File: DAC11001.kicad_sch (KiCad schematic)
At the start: 5 parts

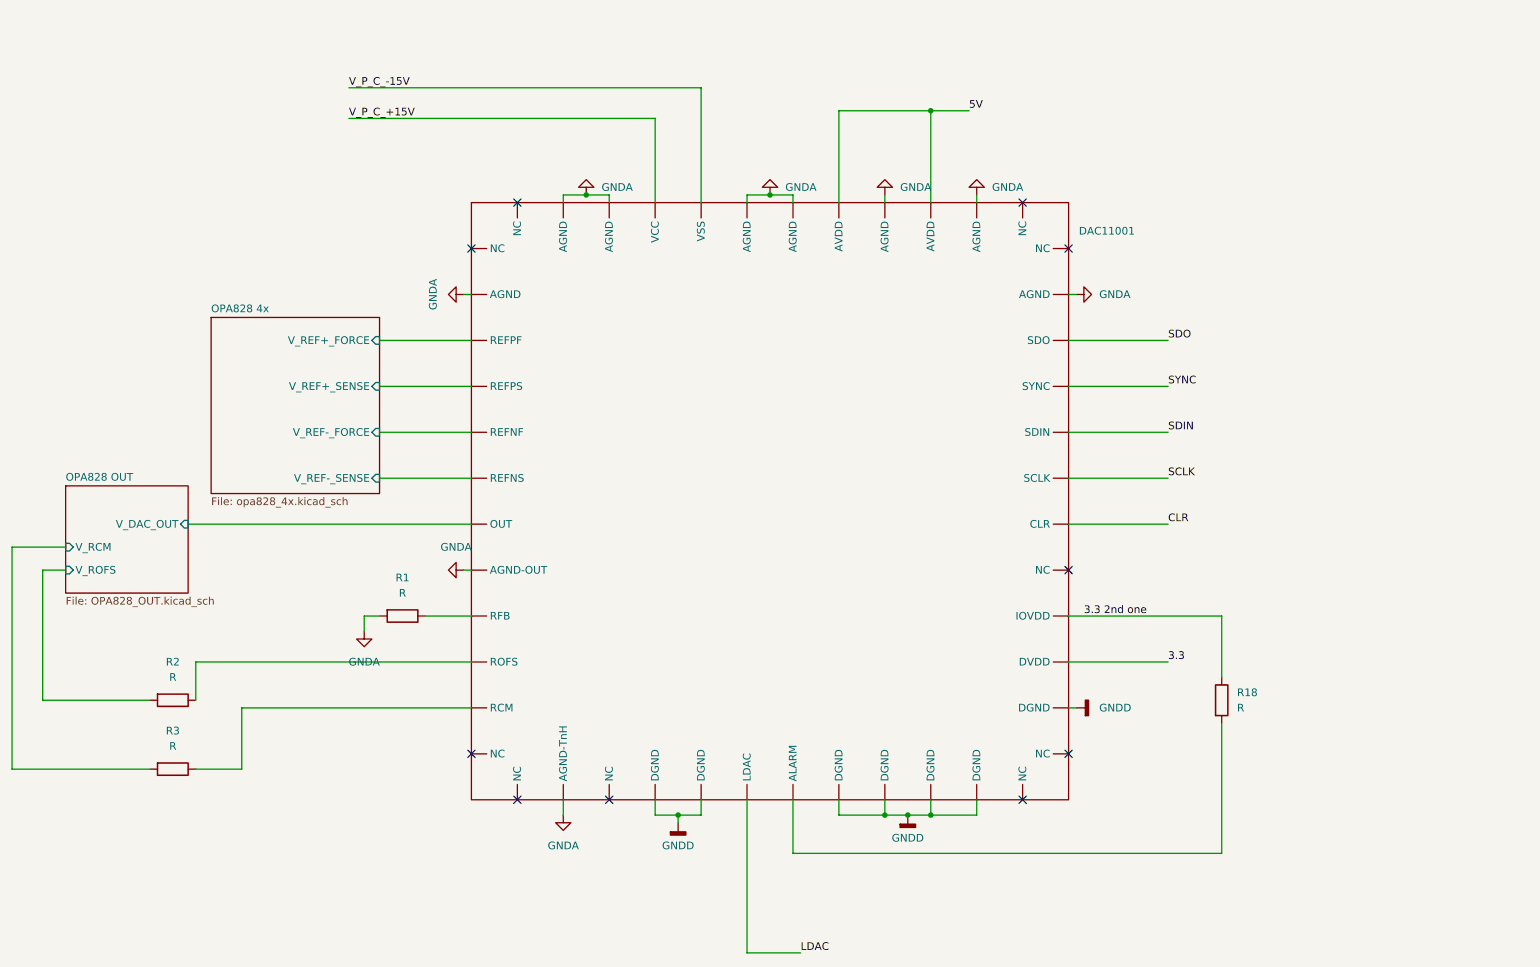
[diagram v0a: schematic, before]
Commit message: done
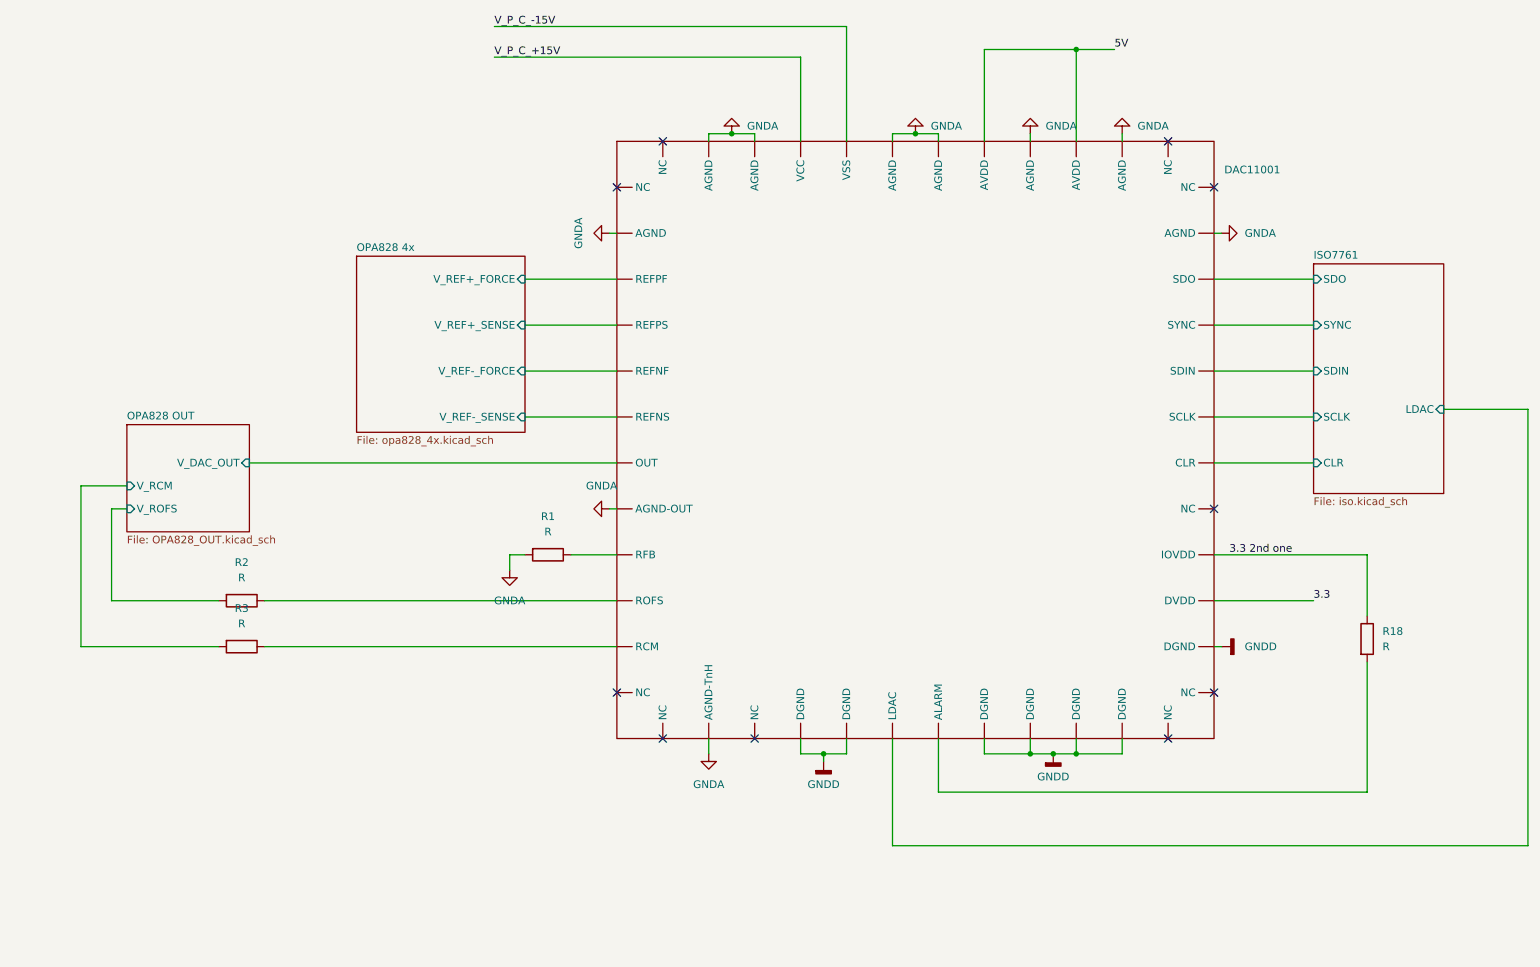
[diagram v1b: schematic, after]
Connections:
- net CLR is gone; now on net V_P_C_-15V: DAC11001. (NC)
- net LDAC is gone; now on net V_P_C_-15V: DAC11001. (NC)
- net SCLK is gone; now on net V_P_C_-15V: DAC11001. (NC)
- net SDIN is gone; now on net V_P_C_-15V: DAC11001. (NC)
- net SDO is gone; now on net V_P_C_-15V: DAC11001. (NC)
- net SYNC is gone; now on net V_P_C_-15V: DAC11001. (NC)
- new net ISO7761/CLR: DAC11001. (NC)
- new net ISO7761/LDAC: DAC11001. (NC)
- new net ISO7761/SCLK: DAC11001. (NC)
- new net ISO7761/SDIN: DAC11001. (NC)
- new net ISO7761/SDO: DAC11001. (NC)
- new net ISO7761/SYNC: DAC11001. (NC)
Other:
- added sheet ISO7761 (iso.kicad_sch)
- moved on the sheet: DAC11001, R1, R18, R2, R3
